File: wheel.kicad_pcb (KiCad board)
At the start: 2 copper layers, 68.5 x 40.5 mm, 11 parts, among them J1 Conn_01x09, SW1 SW_DPST, SW2 SW_DPST, SW3 SW_DPST, SW4 SW_DPST, SW5 SW_DPST, SW6 SW_DPST, SW7 SW_DPST, SW8 SW_DPST

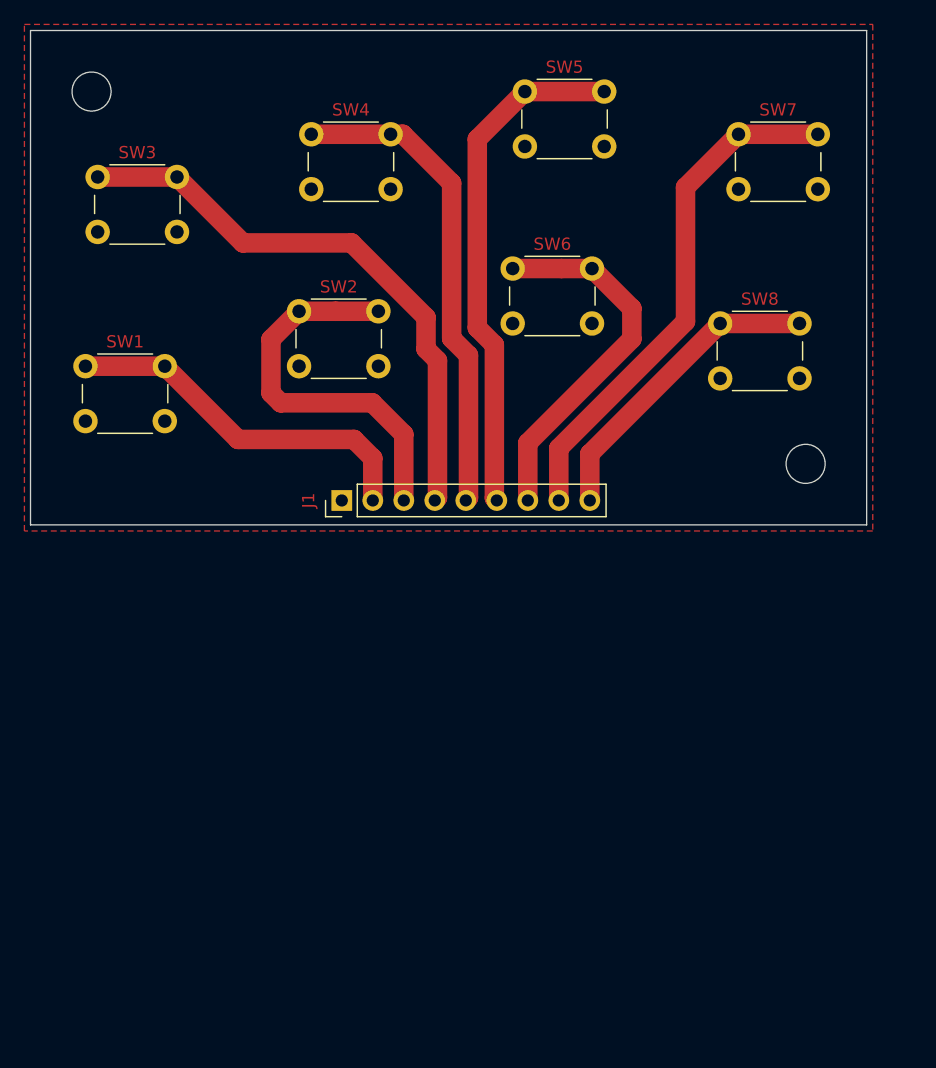
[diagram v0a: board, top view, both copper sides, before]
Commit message: add firmware
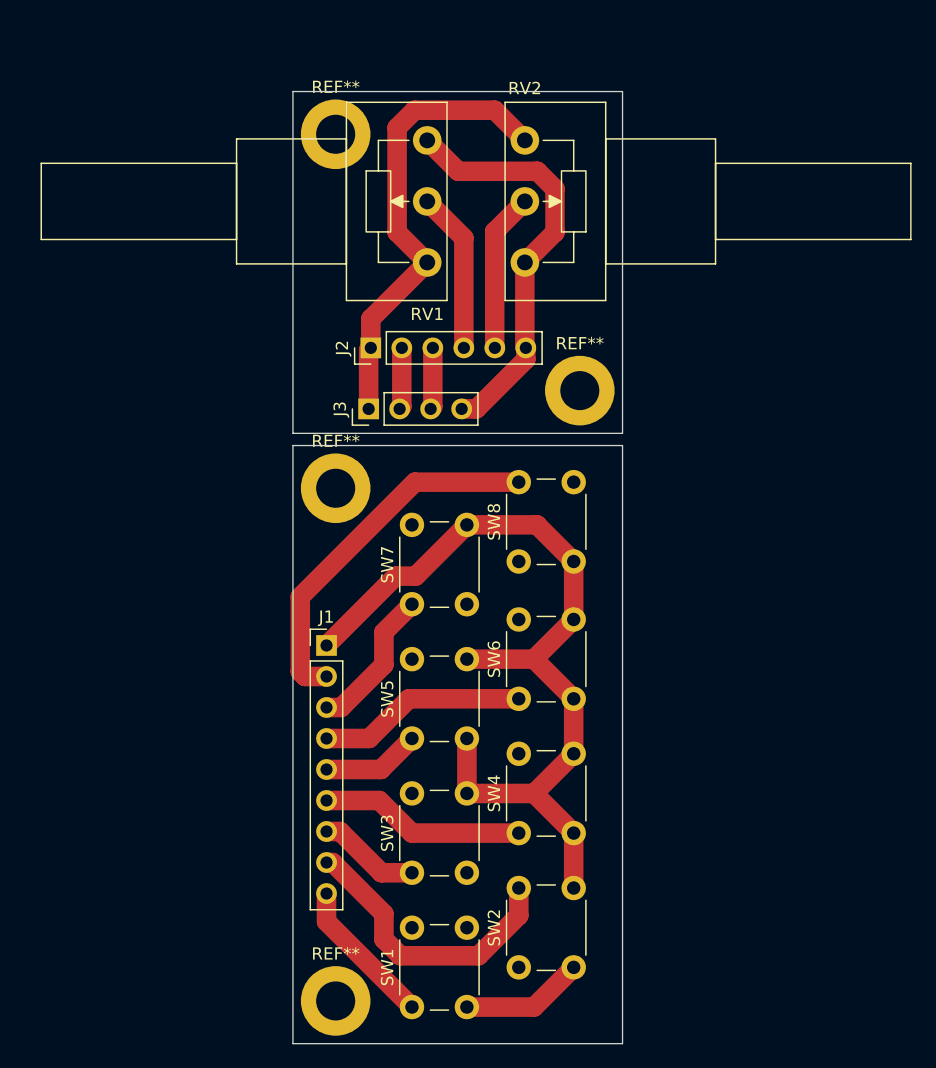
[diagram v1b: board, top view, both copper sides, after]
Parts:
- removed the REF** at (146.0, 90.5)
- removed the REF** at (87.5, 60.0)
- added J2: Conn_01x06_Socket, Connector_PinHeader_2.54mm:PinHeader_1x06_P2.54mm_Vertical, F.Cu at (110.4, 81.0)
- added J3: Conn_01x04_Socket, Connector_PinHeader_2.54mm:PinHeader_1x04_P2.54mm_Vertical, F.Cu at (110.2, 86.0)
- added REF**: MountingHole_3.2mm_M3_ISO7380_Pad, MountingHole:MountingHole_3.2mm_M3_ISO7380_Pad, F.Cu at (127.5, 84.5)
- added REF**: MountingHole_3.2mm_M3_ISO7380_Pad, MountingHole:MountingHole_3.2mm_M3_ISO7380_Pad, F.Cu at (107.5, 92.5)
- added REF**: MountingHole_3.2mm_M3_ISO7380_Pad, MountingHole:MountingHole_3.2mm_M3_ISO7380_Pad, F.Cu at (107.5, 134.5)
- added REF**: MountingHole_3.2mm_M3_ISO7380_Pad, MountingHole:MountingHole_3.2mm_M3_ISO7380_Pad, F.Cu at (107.5, 63.5)
- added RV1: R_Potentiometer, PCM_Potentiometer_THT_AKL:Potentiometer_Piher_PC-16_Single_Horizontal, F.Cu at (115.0, 64.0)
- added RV2: R_Potentiometer, PCM_Potentiometer_THT_AKL:Potentiometer_Piher_PC-16_Single_Horizontal, F.Cu at (123.0, 74.0)
- moved SW3 62.5 mm to (113.8, 124.0), turned to 90 degrees
- moved SW4 59.7 mm to (122.5, 120.8), turned to 90 degrees
- moved SW1 58.9 mm to (113.8, 135.0), turned to 90 degrees
- moved SW2 56.7 mm to (122.5, 131.8), turned to 90 degrees
- moved SW5 53.8 mm to (113.8, 113.0), turned to 90 degrees
- moved SW7 46.9 mm to (113.8, 102.0), turned to 90 degrees
- moved SW6 35.3 mm to (122.5, 109.8), turned to 90 degrees
- moved SW8 25.5 mm to (122.5, 98.5), turned to 90 degrees
- moved J1 11.9 mm to (106.8, 105.4), turned to 0 degrees
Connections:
- J1 pad 2: Net-(J1-Pin_2) -> /Buttons/A
- J1 pad 3: Net-(J1-Pin_3) -> /Buttons/B
- J1 pad 4: Net-(J1-Pin_4) -> /Buttons/X
- J1 pad 5: Net-(J1-Pin_5) -> /Buttons/Y
- J1 pad 6: Net-(J1-Pin_6) -> /Buttons/LB
- J1 pad 7: Net-(J1-Pin_7) -> /Buttons/LT
- J1 pad 8: Net-(J1-Pin_8) -> /Buttons/RB
- J1 pad 9: Net-(J1-Pin_9) -> /Buttons/RT
- SW1 pad 1: Net-(J1-Pin_2) -> /Buttons/RT
- SW2 pad 1: Net-(J1-Pin_3) -> /Buttons/RB
- SW3 pad 1: Net-(J1-Pin_4) -> /Buttons/LT
- SW4 pad 1: Net-(J1-Pin_5) -> /Buttons/LB
- SW5 pad 1: Net-(J1-Pin_6) -> /Buttons/Y
- SW6 pad 1: Net-(J1-Pin_7) -> /Buttons/X
- SW7 pad 1: Net-(J1-Pin_8) -> /Buttons/B
- SW8 pad 1: Net-(J1-Pin_9) -> /Buttons/A
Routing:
- net GND: track 0.00 -> 121.4 mm
- net Net-(J1-Pin_4): track 47.1 -> 0.00 mm
- net Net-(J1-Pin_8): track 42.6 -> 0.00 mm
- net Net-(J1-Pin_6): track 42.3 -> 0.00 mm
- net Net-(J1-Pin_5): track 39.8 -> 0.00 mm
- net 5V: track 0.00 -> 34.1 mm
- net Net-(J1-Pin_3): track 31.9 -> 0.00 mm
- net Net-(J1-Pin_7): track 30.4 -> 0.00 mm
- net /Buttons/A: track 0.00 -> 30.2 mm
- net Net-(J1-Pin_2): track 30.1 -> 0.00 mm
- net Net-(J1-Pin_9): track 25.7 -> 0.00 mm
- net /Buttons/RB: track 0.00 -> 23.8 mm
- net /Buttons/X: track 0.00 -> 17.1 mm
- net /Buttons/LB: track 0.00 -> 16.9 mm
- net Accelerator: track 0.00 -> 13.2 mm
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- removed copper zone on F.Cu, net GND
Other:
- board size 68.5 x 40.5 mm -> 27 x 78 mm
